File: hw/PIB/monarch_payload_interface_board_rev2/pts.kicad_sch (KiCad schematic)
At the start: 17 parts, among them U9 AD7124-8BCPZ-RL

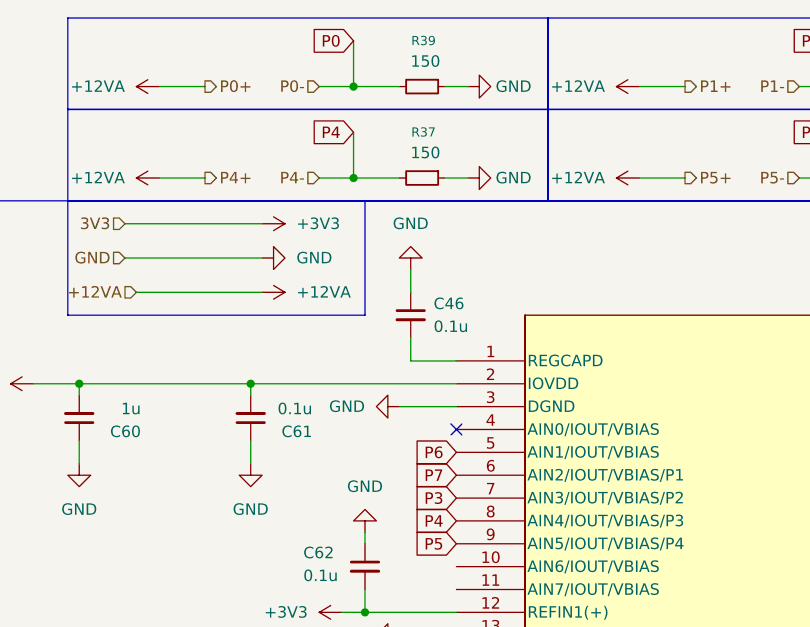
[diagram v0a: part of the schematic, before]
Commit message: AD7124 fixes
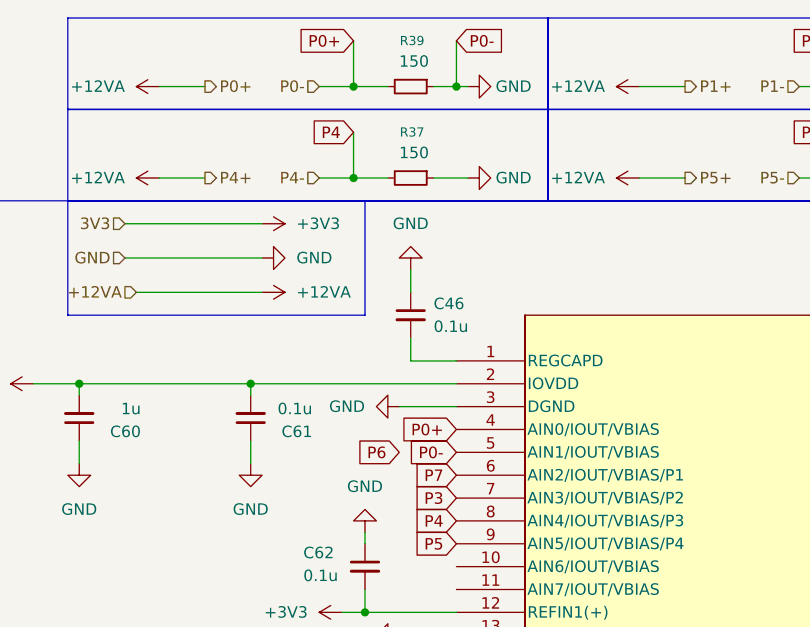
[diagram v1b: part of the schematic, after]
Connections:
- net GND is gone; now on net +12VA: C46.1, C47.1, C60.1, C61.1, C62.1, C63.1, C64.1, C70.2, R32.1, R33.1, R34.1, R35.1, R36.1, R37.1, R38.1, R39.1, U9.13 (REFIN1(-)), U9.23 (AVSS), U9.3 (DGND), U9.33 (EP)
- net +12VA: now also R39.2, U9.4 (AIN0/IOUT/VBIAS), U9.5 (AIN1/IOUT/VBIAS)
- net P0: no longer R39.2
- net P6: no longer U9.5 (AIN1/IOUT/VBIAS)
- no-connect marks 10 -> 9
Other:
- moved on the sheet: R37, R39
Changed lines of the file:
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@@
 	)
 	(junction
-		(at 177.8 30.48)
+		(at 82.55 30.48)
 		(diameter 0)
 		(color 0 0 0 0)
 	)
 	(junction
-		(at 243.84 78.74)
+		(at 177.8 30.48)
 		(diameter 0)
 		(color 0 0 0 0)
 	)
 	(junction
-		(at 71.12 40.64)
+		(at 243.84 78.74)
 		(diameter 0)
 		(color 0 0 0 0)
@@
 	)
 	(junction
-		(at 124.46 40.64)
+		(at 71.12 40.64)
 		(diameter 0)
 		(color 0 0 0 0)
 	)
 	(junction
-		(at 71.12 30.48)
+		(at 124.46 40.64)
 		(diameter 0)
 		(color 0 0 0 0)
@@
 	)
 	(junction
+		(at 71.12 30.48)
+		(diameter 0)
+		(color 0 0 0 0)
+	)
+	(junction
 		(at 231.14 40.64)
 		(diameter 0)
@@
 	)
 	(no_connect
-		(at 82.55 68.58)
-	)
-	(no_connect
 		(at 82.55 96.52)
 	)
@@
 	(wire
 		(pts
+			(xy 82.55 30.48) (xy 83.82 30.48)
+		)
+		(stroke
+			(width 0)
+			(type default)
+		)
+	)
+	(wire
+		(pts
 			(xy 243.84 78.74) (xy 248.92 78.74)
 		)
@@
 	(wire
 		(pts
+			(xy 82.55 25.4) (xy 82.55 30.48)
+		)
+		(stroke
+			(width 0)
+			(type default)
+		)
+	)
+	(wire
+		(pts
 			(xy 199.39 68.58) (xy 204.47 68.58)
 		)
@@
 	(wire
 		(pts
-			(xy 71.12 30.48) (xy 76.2 30.48)
+			(xy 71.12 30.48) (xy 74.93 30.48)
 		)
 		(stroke
@@
 	(wire
 		(pts
-			(xy 81.28 30.48) (xy 83.82 30.48)
+			(xy 80.01 30.48) (xy 82.55 30.48)
 		)
 		(stroke
@@
 	(wire
 		(pts
-			(xy 71.12 40.64) (xy 76.2 40.64)
+			(xy 71.12 40.64) (xy 74.93 40.64)
 		)
 		(stroke
@@
 	(wire
 		(pts
-			(xy 81.28 40.64) (xy 83.82 40.64)
+			(xy 80.01 40.64) (xy 83.82 40.64)
 		)
 		(stroke
@@
 		)
 	)
+	(global_label "P0-"
+		(shape input)
+		(at 82.55 25.4 0)
+		(fields_autoplaced yes)
+		(effects
+			(font
+				(size 1.27 1.27)
+			)
+			(justify left)
+		)
+		(property "Intersheetrefs" "${INTERSHEET_REFS}"
+			(at 88.9329 25.4 0)
+			(hide yes)
+			(show_name no)
+			(do_not_autoplace no)
+			(effects
+				(font
+					(size 1.27 1.27)
+				)
+				(justify left)
+			)
+		)
+	)
 	(global_label "P1"
 		(shape input)
@@
 		)
 	)
+	(global_label "P0+"
+		(shape input)
+		(at 82.55 68.58 180)
+		(fields_autoplaced yes)
+		(effects
+			(font
+				(size 1.27 1.27)
+			)
+			(justify right)
+		)
+		(property "Intersheetrefs" "${INTERSHEET_REFS}"
+			(at 76.1671 68.58 0)
+			(hide yes)
+			(show_name no)
+			(do_not_autoplace no)
+			(effects
+				(font
+					(size 1.27 1.27)
+				)
+				(justify right)
+			)
+		)
+	)
 	(global_label "P6"
 		(shape input)
-		(at 82.55 71.12 180)
+		(at 76.2 71.12 180)
 		(fields_autoplaced yes)
 		(effects
@@
 		)
 		(property "Intersheetrefs" "${INTERSHEET_REFS}"
-			(at 77.0853 71.12 0)
+			(at 70.7353 71.12 0)
 			(hide yes)
 			(show_name no)
@@
 		)
 	)
-	(global_label "P0"
+	(global_label "P0-"
+		(shape input)
+		(at 82.55 71.12 180)
+		(fields_autoplaced yes)
+		(effects
+			(font
+				(size 1.27 1.27)
+			)
+			(justify right)
+		)
+		(property "Intersheetrefs" "${INTERSHEET_REFS}"
+			(at 76.1671 71.12 0)
+			(hide yes)
+			(show_name no)
+			(do_not_autoplace no)
+			(effects
+				(font
+					(size 1.27 1.27)
+				)
+				(justify right)
+			)
+		)
+	)
+	(global_label "P0+"
 		(shape input)
 		(at 71.12 25.4 180)
@@
 		)
 		(property "Intersheetrefs" "${INTERSHEET_REFS}"
-			(at 65.6553 25.4 0)
+			(at 64.7371 25.4 0)
 			(hide yes)
 			(show_name no)
@@
 	(symbol
 		(lib_id "Device:R_Small")
-		(at 78.74 30.48 270)
+		(at 77.47 30.48 270)
 		(unit 1)
 		(body_style 1)
@@
 		(dnp no)
 		(property "Reference" "R39"
-			(at 80.264 25.4 90)
+			(at 78.994 25.4 90)
 			(show_name no)
 			(do_not_autoplace no)
@@
 		)
 		(property "Value" "150"
-			(at 80.772 27.686 90)
+			(at 79.502 27.686 90)
 			(show_name no)
 			(do_not_autoplace no)
@@
 		)
 		(property "Footprint" "Resistor_SMD:R_0603_1608Metric"
-			(at 78.74 30.48 0)
+			(at 77.47 30.48 0)
 			(hide yes)
 			(show_name no)
@@
 		)
 		(property "Datasheet" ""
-			(at 78.74 30.48 0)
+			(at 77.47 30.48 0)
 			(hide yes)
 			(show_name no)
@@
 		)
 		(property "Description" "Resistor, small symbol"
-			(at 78.74 30.48 0)
+			(at 77.47 30.48 0)
 			(hide yes)
 			(show_name no)
@@
 	(symbol
 		(lib_id "Device:R_Small")
-		(at 78.74 40.64 270)
+		(at 77.47 40.64 270)
 		(unit 1)
 		(body_style 1)
@@
 		(dnp no)
 		(property "Reference" "R37"
-			(at 80.264 35.56 90)
+			(at 78.994 35.56 90)
 			(show_name no)
 			(do_not_autoplace no)
@@
 		)
 		(property "Value" "150"
-			(at 80.772 37.846 90)
+			(at 79.502 37.846 90)
 			(show_name no)
 			(do_not_autoplace no)
@@
 		)
 		(property "Footprint" "Resistor_SMD:R_0603_1608Metric"
-			(at 78.74 40.64 0)
+			(at 77.47 40.64 0)
 			(hide yes)
 			(show_name no)
@@
 		)
 		(property "Datasheet" ""
-			(at 78.74 40.64 0)
+			(at 77.47 40.64 0)
 			(hide yes)
 			(show_name no)
@@
 		)
 		(property "Description" "Resistor, small symbol"
-			(at 78.74 40.64 0)
+			(at 77.47 40.64 0)
 			(hide yes)
 			(show_name no)
